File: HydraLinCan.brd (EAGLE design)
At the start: 59.9 x 37 mm, 33 parts, among them CN1 8p-2.54, J1 HYDRABUS_SHIELD_CON_HEADER_2X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, J2 HYDRABUS_SHIELD_CON_HEADER_2X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, J3 HYDRABUS_SHIELD_CON_HEADER_2X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, K1 TS-1188E, U1 SN65HVD233DG4, U2 SN65HVD233DG4, U3 CJ78M05-to252

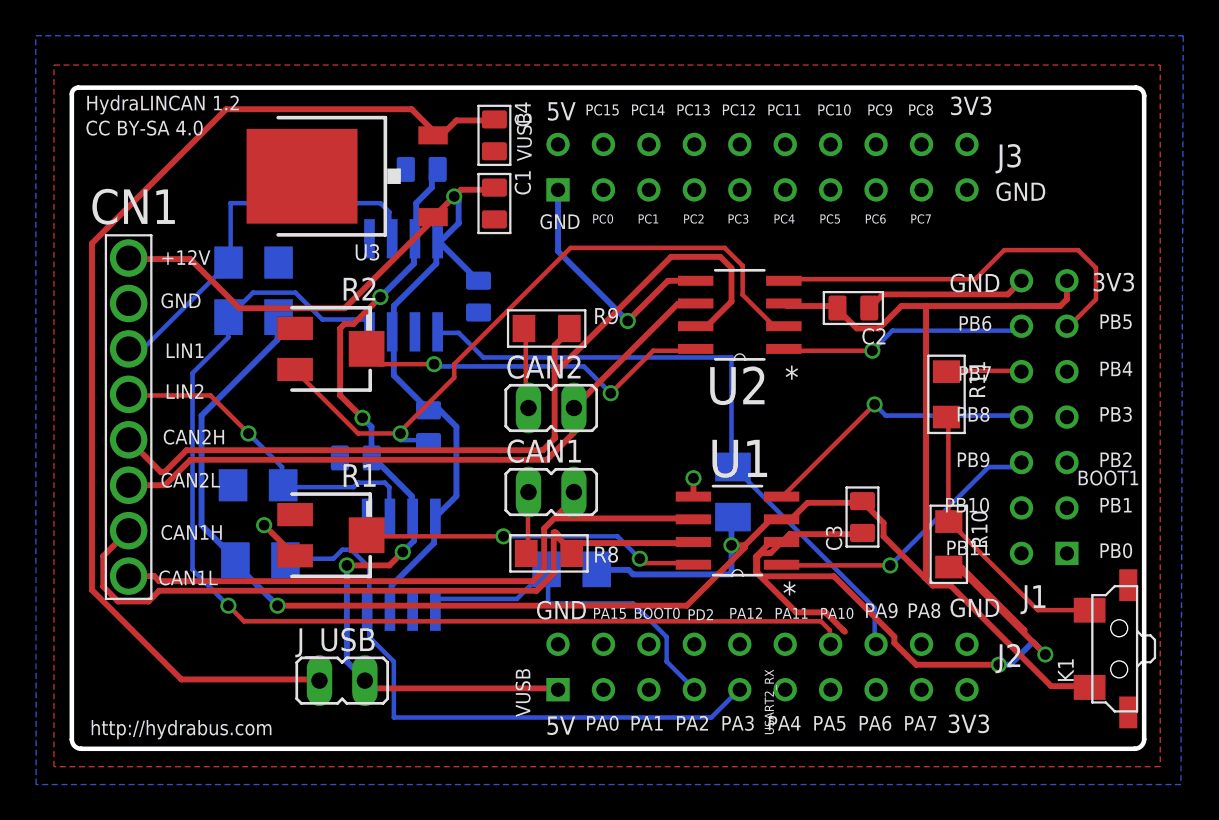
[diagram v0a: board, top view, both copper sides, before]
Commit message: Silkscreen cleaning
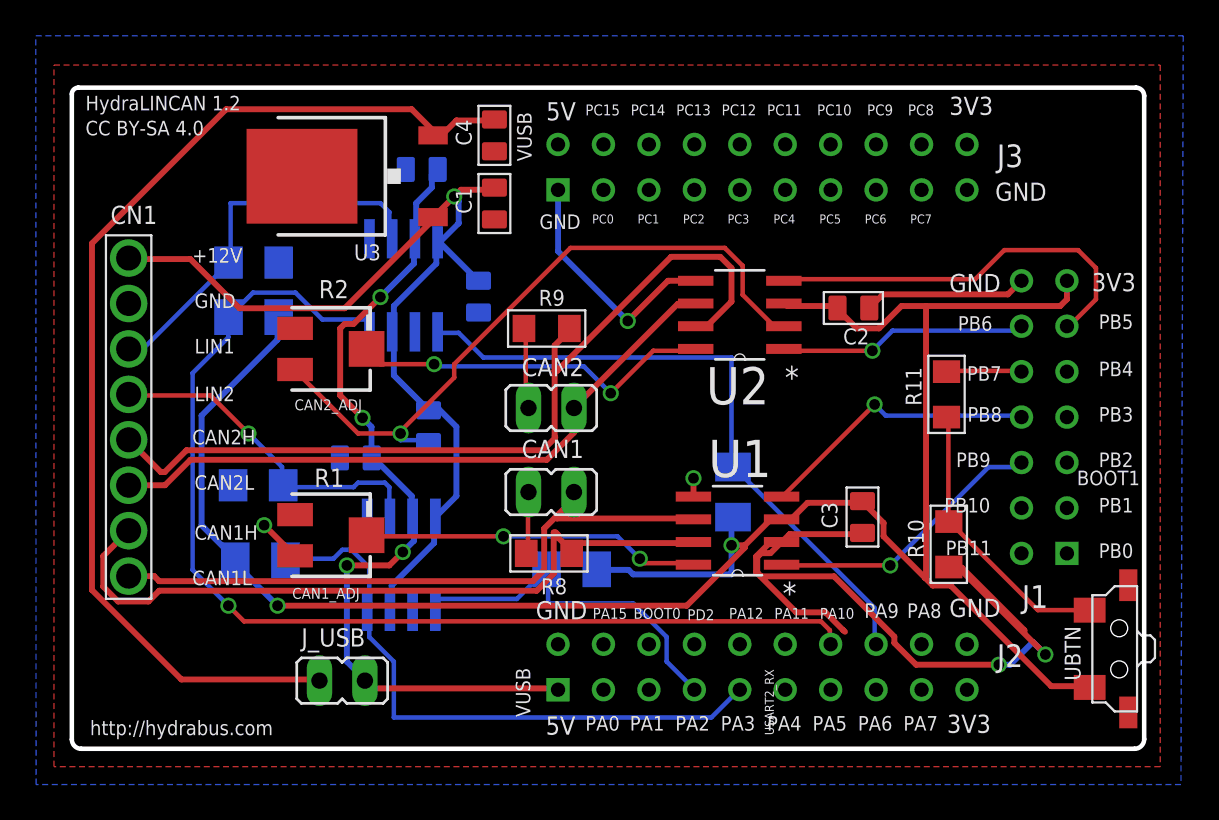
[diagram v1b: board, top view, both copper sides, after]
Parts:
- renumbered K1 to UBTN
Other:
- board text added: "CAN1_ADJ"
- board text added: "CAN2_ADJ"
